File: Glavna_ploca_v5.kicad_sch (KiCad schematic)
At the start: 85 parts, among them J1 PUMPA1, J10 Granicni prekidac gl, J11 Granicni prekidac gd, J12 Senzor dp, J13 Senzor dz, J14 Senzor gzl, J15 Senzor gzd, J16 Senzor gnl, J17 Senzor gnd, J18 Prekidac za boje, J19 Prekidac za strategije, J2 PUMPA ZA DASKE, J20 Enkoder levi, J21 Enkoder desni, J22 Cinc, J23 Servo, J24 LCD, J25 12V, J26 5V, J27 TMC2209_1, J28 TMC2209_2, J3 PUMPA2, J4 PUMPA3, J5 PUMPA4, J6 Granicni prekidac id, J7 Granicni prekidac il, J8 Granicni prekidac dl, J9 Granicni prekidac dd, Q1 IRLZ44N, Q2 IRLZ44N, Q3 IRLZ44N, Q4 IRLZ44N, Q5 IRLZ44N, U1 NUCLEO-F401RE, U2 TMC2209, U3 TMC2209

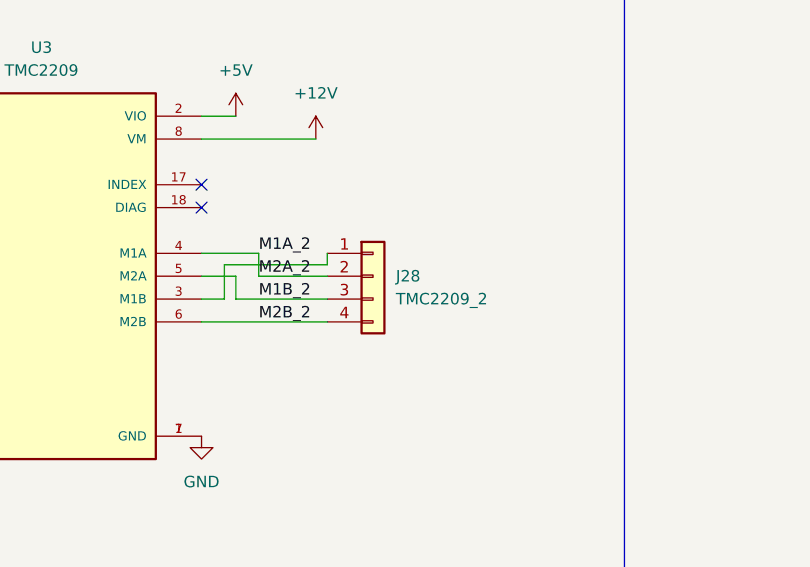
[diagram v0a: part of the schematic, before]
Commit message: konacna ploca
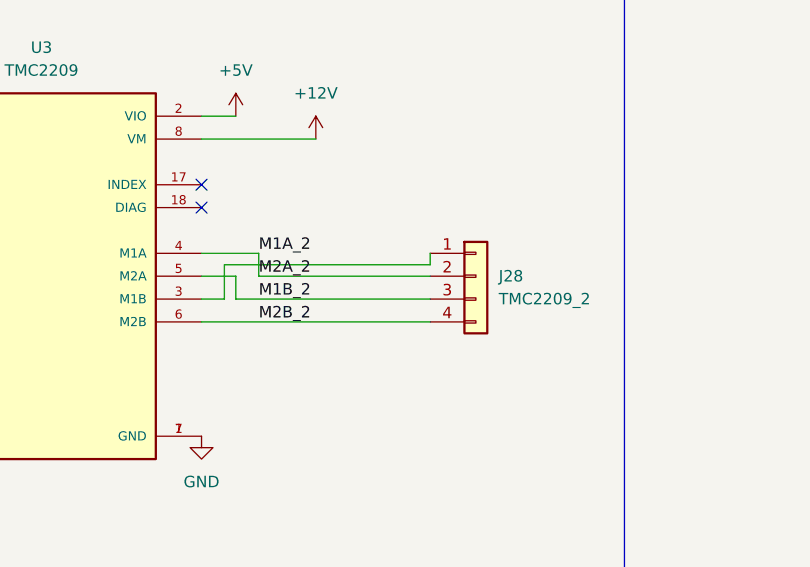
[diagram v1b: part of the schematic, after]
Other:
- moved on the sheet: J28
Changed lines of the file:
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@@
 	(wire
 		(pts
-			(xy 293.37 140.97) (xy 307.34 140.97)
+			(xy 293.37 140.97) (xy 318.77 140.97)
 		)
 		(stroke
@@
 	(wire
 		(pts
-			(xy 297.18 138.43) (xy 307.34 138.43)
+			(xy 297.18 138.43) (xy 318.77 138.43)
 		)
 		(stroke
@@
 	(wire
 		(pts
-			(xy 299.72 135.89) (xy 307.34 135.89)
+			(xy 299.72 135.89) (xy 318.77 135.89)
 		)
 		(stroke
@@
 	(wire
 		(pts
-			(xy 295.91 134.62) (xy 307.34 134.62)
+			(xy 295.91 134.62) (xy 318.77 134.62)
 		)
 		(stroke
@@
 	(wire
 		(pts
-			(xy 307.34 134.62) (xy 307.34 133.35)
+			(xy 318.77 134.62) (xy 318.77 133.35)
 		)
 		(stroke
@@
 	(symbol
 		(lib_id "Connector_Generic:Conn_01x04")
-		(at 312.42 135.89 0)
+		(at 323.85 135.89 0)
 		(unit 1)
 		(exclude_from_sim no)
@@
 		(fields_autoplaced yes)
 		(property "Reference" "J28"
-			(at 314.96 135.8899 0)
+			(at 326.39 135.8899 0)
 			(effects
 				(font
@@
 		)
 		(property "Value" "TMC2209_2"
-			(at 314.96 138.4299 0)
+			(at 326.39 138.4299 0)
 			(effects
 				(font
@@
 		)
 		(property "Footprint" "Connector_JST:JST_XH_B4B-XH-A_1x04_P2.50mm_Vertical"
-			(at 312.42 135.89 0)
+			(at 323.85 135.89 0)
 			(effects
 				(font
@@
 		)
 		(property "Datasheet" "~"
-			(at 312.42 135.89 0)
+			(at 323.85 135.89 0)
 			(effects
 				(font
@@
 		)
 		(property "Description" "Generic connector, single row, 01x04, script generated (kicad-library-utils/schlib/autogen/connector/)"
-			(at 312.42 135.89 0)
+			(at 323.85 135.89 0)
 			(effects
 				(font
